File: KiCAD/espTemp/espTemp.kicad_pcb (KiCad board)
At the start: 2 copper layers, 36.2 x 23.5 mm, 7 parts, among them U1 ESP-01, U2 LD1117S33TR_SOT223, U3 DHT22,CM2303

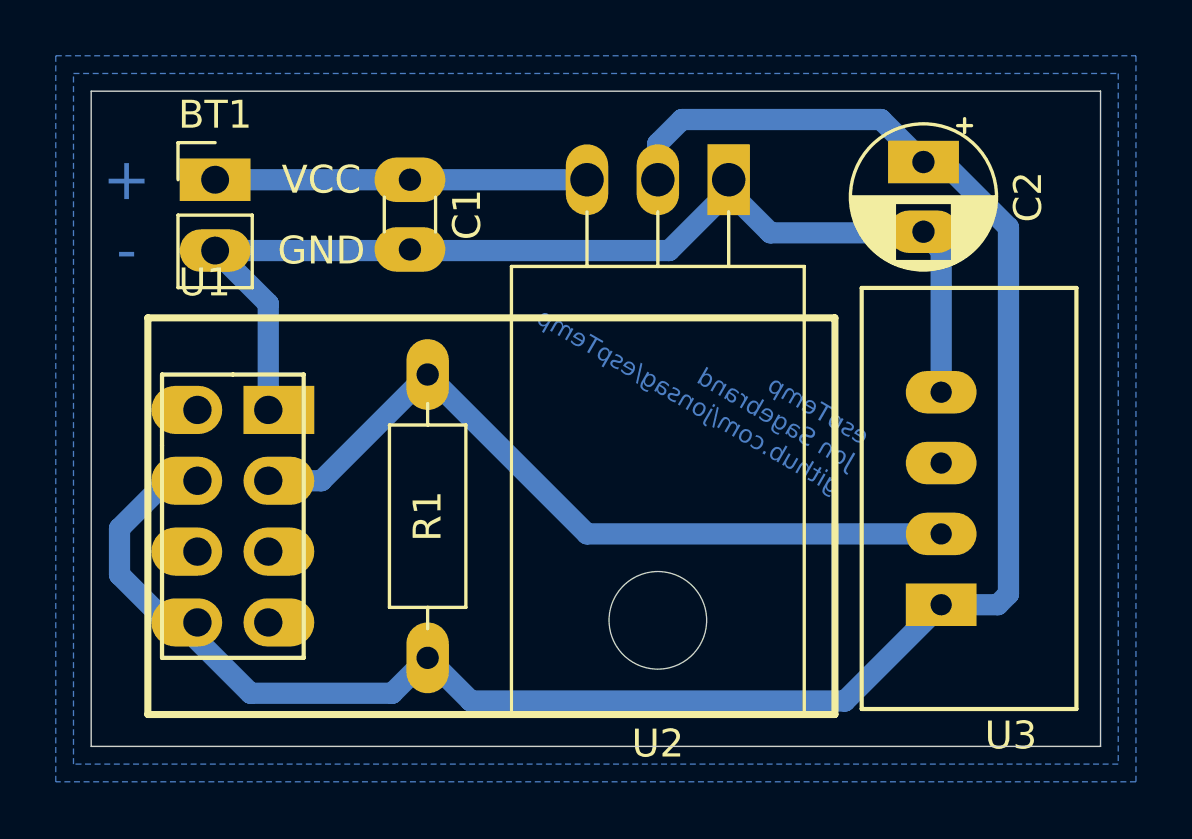
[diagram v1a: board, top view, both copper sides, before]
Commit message: 3d view
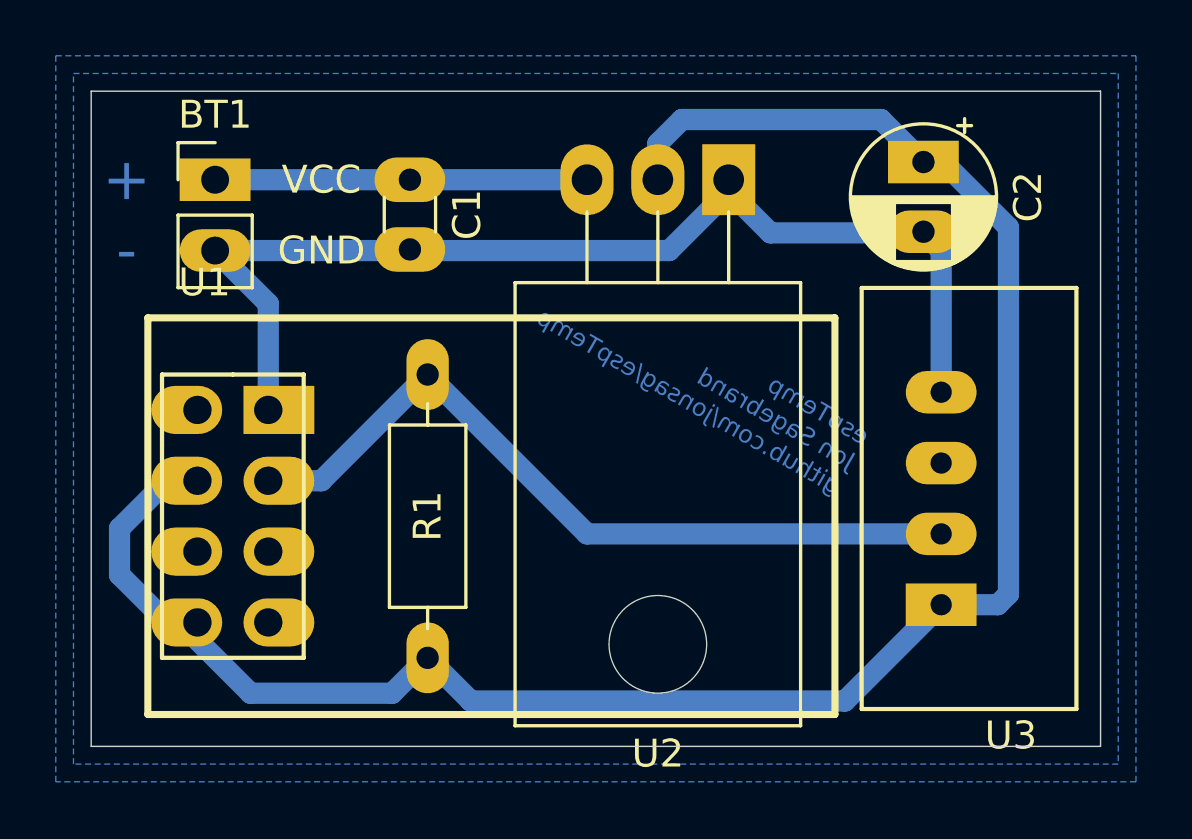
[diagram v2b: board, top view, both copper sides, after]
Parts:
- U1: footprint My_Arduino:ESP-01_large -> My_Arduino:ESP-01_w_pin_socket_large
- U2: footprint My_Misc:TO-220F-3_Horizontal_TabDown_large -> My_Misc:TO-220-3_Horizontal_TabDown_large
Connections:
- net GPIO2 renamed TempSignal
- U3 pad 3: Net-(U3-Pad3) -> unconnected-(U3-Pad3)
